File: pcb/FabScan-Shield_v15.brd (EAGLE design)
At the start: 68.6 x 53.3 mm, 44 parts, among them T1A BC547, T1B IRLML2502, X1 PASSER, X2 PASSER, X3 PASSER

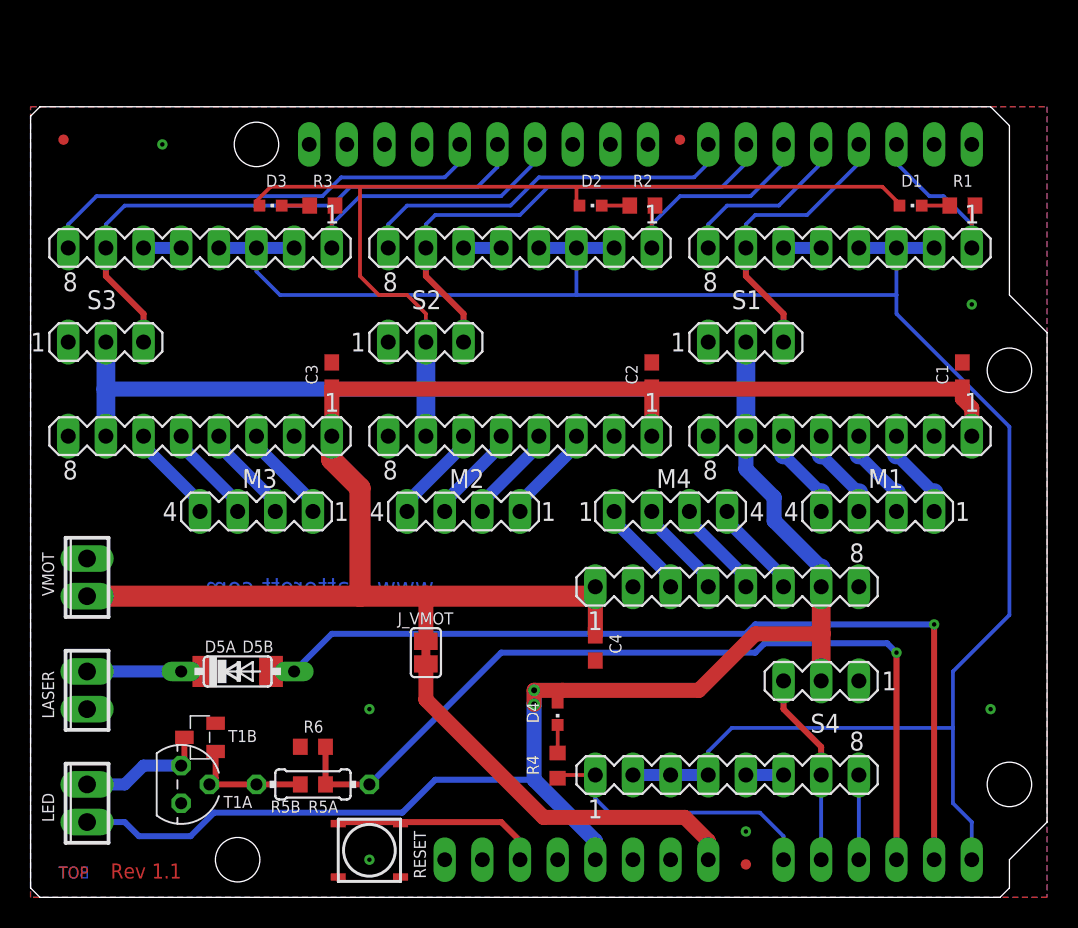
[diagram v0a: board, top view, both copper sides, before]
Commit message: updated layout and schematics
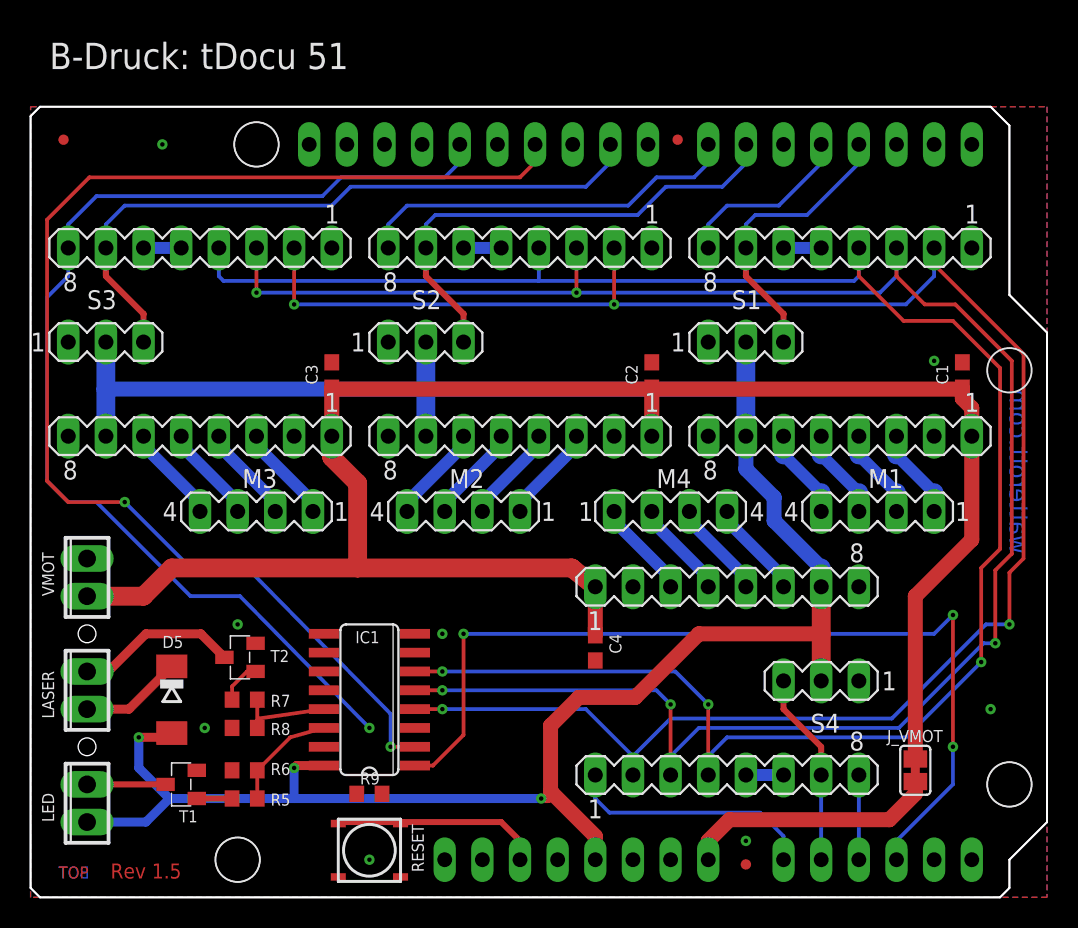
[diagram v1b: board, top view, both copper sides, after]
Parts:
- removed A1: UNO, Arduino:UNO
- removed D1, D2, D3, D4: (no value), led:CHIPLED_0603
- removed D5A: 1N4148, diode:DO35-7
- removed D5B: 1N4148, diode:SOD106-R
- removed R1, R2, R3, R4: 1k, rcl:R0603
- removed R5A: 4k7, rcl:0204/7
- removed R5B: 4k7, rcl:R0603
- removed T1A: BC547, transistor:TO92
- removed T1B: IRLML2502, IRF-sot23:MICRO3
- added ARD1: UNOTP, Arduino:UNOTP
- added D5: 1N4148, diode:SOD106-R
- added IC1: 4094D, 40xx:SO16
- added R5, R7: 4k7, rcl:R0603
- added R8, R9: 47k, rcl:R0603
- added T1, T2: IRLML2502, IRF-sot23:MICRO3
- moved J_VMOT 34.0 mm to (59.7, 8.57)
- moved R6 4.87 mm to (14.4, 8.57)
- moved X3 0.16 mm to (43.7, 51.1)
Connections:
- removed net MS: A1.AIN5, D1A.2, D1A.3, D1A.4, D2A.2, D2A.3, D2A.4, D3A.2, D3A.3, D3A.4, D4A.2, D4A.3, D4A.4
- removed net N$2: D1.C, R1.2
- removed net N$3: D2.C, R2.2
- removed net N$4: D3.C, R3.2
- removed net N$7: D4.C, R4.2
- new net EN: ARD1.9, IC1.15, R9.1
- new net MOSI: ARD1.11, IC1.2
- new net MS1: D1A.2, D2A.2, D3A.2, D4A.2, IC1.4
- new net MS2: D1A.3, D2A.3, D3A.3, D4A.3, IC1.5
- new net MS3: D1A.4, D2A.4, D3A.4, D4A.4, IC1.6
- new net N$10: D5.C, LASER.1
- new net N$9: R7.1, T2.1
- new net SCK: ARD1.13, IC1.3
- new net STR: ARD1.8, IC1.1
- net 3V3: now also ARD1.3V3; no longer A1.3V3
- net 5V: now also ARD1.5V, D5.A, IC1.16; no longer A1.5V, D1.A, D2.A, D3.A, D4.A
- net AREF: now also ARD1.AREF; no longer A1.AREF
- net A_DIR: now also ARD1.3; no longer A1.4
- net A_EN: now also IC1.7; no longer A1.2, R1.1
- net A_STEP: now also ARD1.2; no longer A1.3
- net B_DIR: now also ARD1.5; no longer A1.7
- net B_EN: now also IC1.11; no longer A1.5, R2.1
- net B_STEP: now also ARD1.4; no longer A1.6
- net C_DIR: now also ARD1.7; no longer A1.13
- net C_EN: now also IC1.12; no longer A1.11, R3.1
- net C_STEP: now also ARD1.6; no longer A1.12
- net D_DIR: now also ARD1.AIN2; no longer A1.AIN2
- net D_EN: now also ARD1.AIN0; no longer A1.AIN0, R4.1
- net D_STEP: now also ARD1.AIN1; no longer A1.AIN1
- net GND: now also ARD1.GND@1, ARD1.GND@2, ARD1.GND@3, IC1.8, R8.2, R9.2, T1.2, T2.2; no longer A1.GND@1, A1.GND@2, A1.GND@3, LASER.1, T1A.1, T1B.2
- net IOREF: now also ARD1.IOREF; no longer A1.IOREF
- net LASER: now also IC1.13, R7.2, R8.1; no longer A1.AIN4, D5A.A, D5B.A
- net LED: now also IC1.14, R5.2; no longer A1.AIN3, R5A.1, R5B.2
- net N$1: now also T2.3; no longer D5A.C, D5B.C
- net N$6: now also T1.3; no longer T1A.3, T1B.3
- net N$8: now also R5.1, T1.1; no longer R5A.2, R5B.1, T1A.2, T1B.1
- net RST: now also ARD1.RST; no longer A1.RST
- net VIN: now also ARD1.VIN; no longer A1.VIN
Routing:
- net MS: track 134.2 -> 0.00 mm
- net MS2: track 0.00 -> 131.9 mm, vias 0 -> 5
- net MS3: track 0.00 -> 131.6 mm, vias 0 -> 3
- net MS1: track 0.00 -> 128.2 mm, vias 0 -> 4
- net MOSI: track 0.00 -> 87.0 mm, vias 0 -> 2
- net STR: track 0.00 -> 61.3 mm, vias 0 -> 3
- net LASER: track 61.9 -> 7.02 mm, vias 1 -> 0
- net 5V: track 208.8 -> 155.6 mm, vias 2 -> 3
- net LED: track 59.2 -> 7.40 mm, vias 1 -> 0
- net C_DIR: track 30.9 -> 74.7 mm, vias 0 -> 1
- net C_EN: track 21.3 -> 0.00 mm
- net VMOT: track 104.9 -> 124.5 mm
- net B_EN: track 15.3 -> 0.00 mm
- net A_EN: track 12.7 -> 0.00 mm
- net VIN: track 26.7 -> 17.4 mm
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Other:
- board text added: "B-Druck: tDocu 51"
- board text added: "Rev 1.5"
- board text added: "watterott.com"
- board text removed: "Rev 1.1"
- board text removed: "Silkscreen: 51 tDocu"
- board text removed: "www.watterott.com"
